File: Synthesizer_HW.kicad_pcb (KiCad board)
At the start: 2 copper layers, 59.5 x 39 mm, 127 parts, among them J1 +5V_DC, J1&1 Selector, J2 USB_B_Micro, J3 EXT_REF_IN, J4 RF OUT1, J5 RF OUT2, J6 SWD, Q1 BC857, Q2 BC847, Q3 BC847, Q4 IRLML5203, Q5 IRLML5203, U1 USBLC6-2, U2 SN74LVC1G3157, U3 STM32F042F6Px, U4 MAX2871, U5 GVA-63+, U6 XX1002-QH, U7 LT3042xMSE, U8 LP5907MFX-3.3, X1 TXETALSANF-10MHz

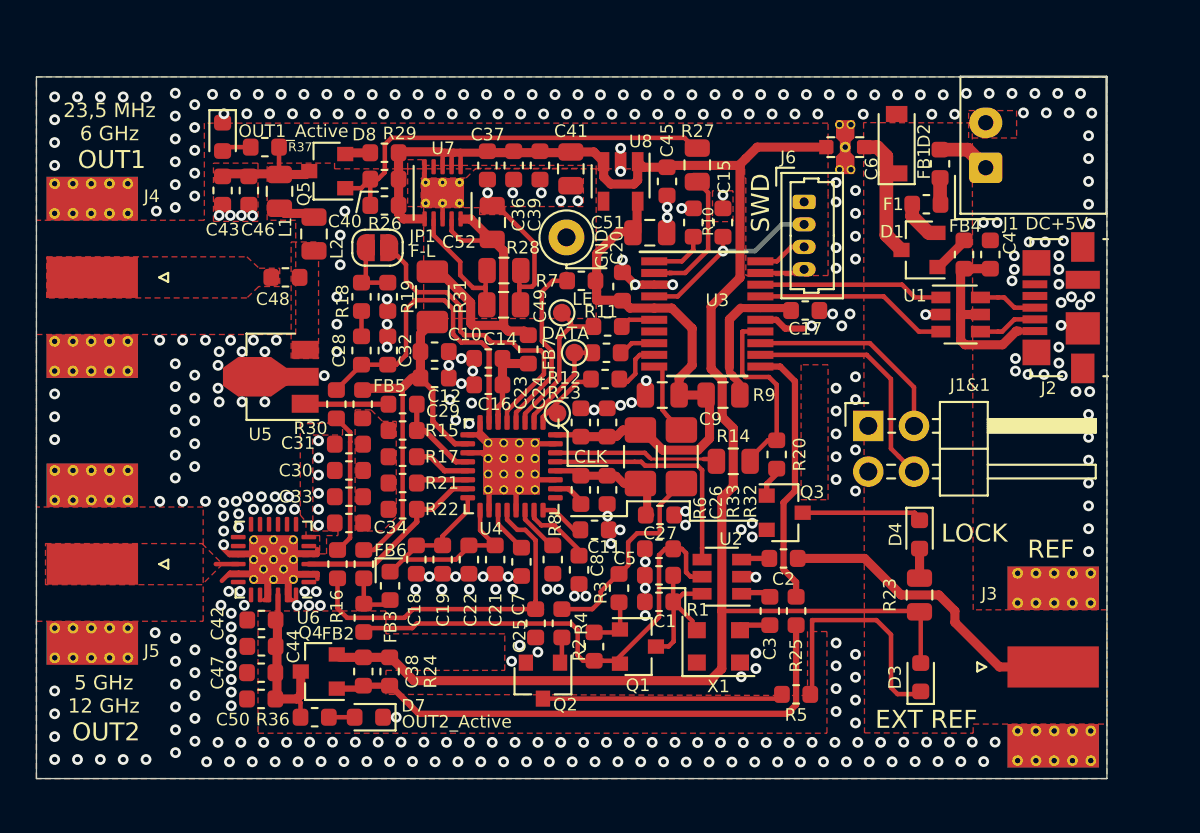
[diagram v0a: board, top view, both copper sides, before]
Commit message: latest vers., after correc., added moun. holes
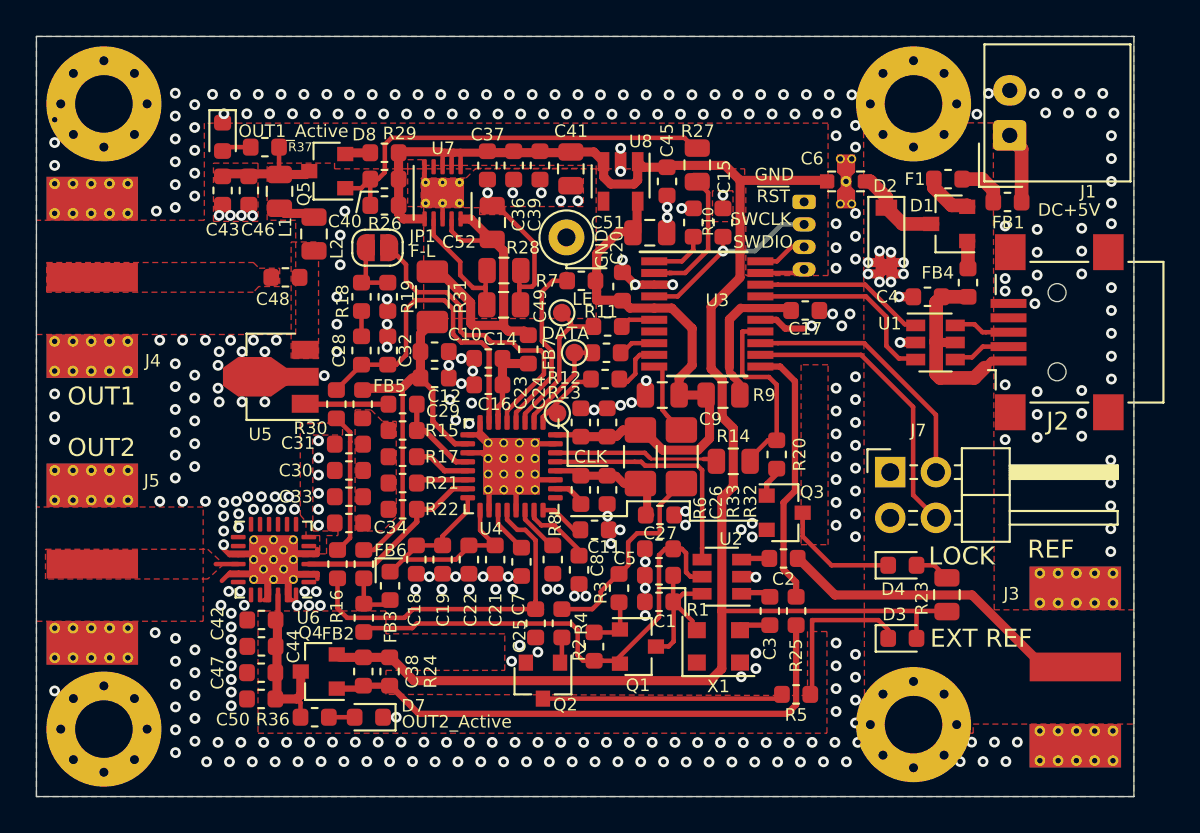
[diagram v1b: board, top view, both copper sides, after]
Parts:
- added H1: MountingHole_Pad, MountingHole:MountingHole_3.2mm_M3_Pad_Via, F.Cu at (102.8, 47.0)
- added H2: MountingHole_Pad, MountingHole:MountingHole_3.2mm_M3_Pad_Via, F.Cu at (147.8, 47.0)
- added H3: MountingHole_Pad, MountingHole:MountingHole_3.2mm_M3_Pad_Via, F.Cu at (147.8, 81.5)
- added H4: MountingHole_Pad, MountingHole:MountingHole_3.2mm_M3_Pad_Via, F.Cu at (102.8, 81.8)
- J2: value USB_B_Micro -> USB_B_Mini; footprint Connector_USB:USB_Micro-B_Molex_47346-0001 -> Connector_USB:USB_Mini-B_Lumberg_2486_01_Horizontal
- J6: moved to B.Cu
- moved D2 5.24 mm to (146.2, 54.4), turned to -90 degrees
- moved FB1 4.31 mm to (153.0, 52.5), turned to 0 degrees
- moved C4 4.21 mm to (148.5, 57.7), turned to 180 degrees
- moved J7 2.85 mm to (146.5, 67.5)
- moved D3 2.39 mm to (147.1, 76.7), turned to 0 degrees
- moved J1 2.24 mm to (153.1, 48.8)
- moved D1 2.20 mm to (149.7, 53.7)
- moved U1 2.09 mm to (149.0, 60.3)
- moved D4 1.96 mm to (147.1, 72.6), turned to 0 degrees
- moved C6 1.91 mm to (144.0, 51.3)
- moved F1 1.85 mm to (149.7, 51.2)
- moved FB4 1.58 mm to (150.8, 56.9)
- moved R23 1.52 mm to (149.6, 74.3)
- moved J2 1.38 mm to (155.7, 59.7)
- moved J3 1.23 mm to (155.0, 78.3)
- renumbered J1&1 to J7
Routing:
- net GND: track 54.1 -> 63.3 mm, vias 391 -> 380
- net Net-(D3-Pad1): track 13.7 -> 9.10 mm
- net Net-(J1&1-Pad4): track 13.5 -> 16.8 mm
- net Net-(J1&1-Pad2): track 11.7 -> 14.6 mm
- net Net-(C6-Pad1): track 7.55 -> 5.02 mm
- net Net-(F1-Pad2): track 1.47 -> 2.64 mm
- net /USB_D+: track 10.4 -> 9.54 mm
- net Net-(C2-Pad2): track 17.2 -> 17.9 mm
- net Net-(D1-Pad1): track 2.07 -> 1.54 mm
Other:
- board size 59.5 x 39 mm -> 61 x 42.2 mm
- board text added: "~RST"
- board text removed: "23,5 MHz 6 GHz"
- board text removed: "5 GHz 12 GHz"
- board text removed: "~CLK"
